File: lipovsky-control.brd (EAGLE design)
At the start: 59 x 32 mm, 31 parts, among them J1 M04-929P, J2 M04-929P, J3 M04-929P, J4 M04-929P, U1 ATTINYX4A8MU, U10 CCR20MA_45V, U2 MIC2288YD5, U3 MIC2288YD5, U7 LTV-816S

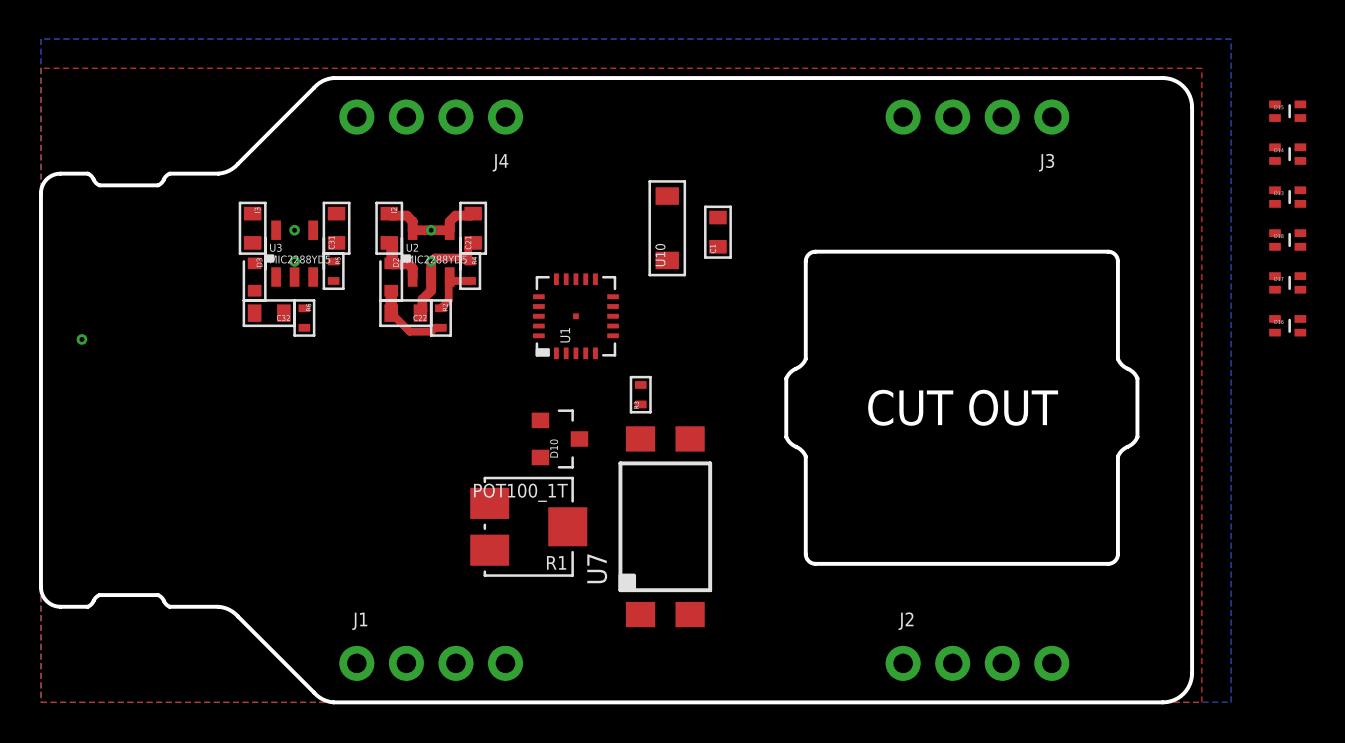
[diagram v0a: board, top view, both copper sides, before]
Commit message: LED matrix
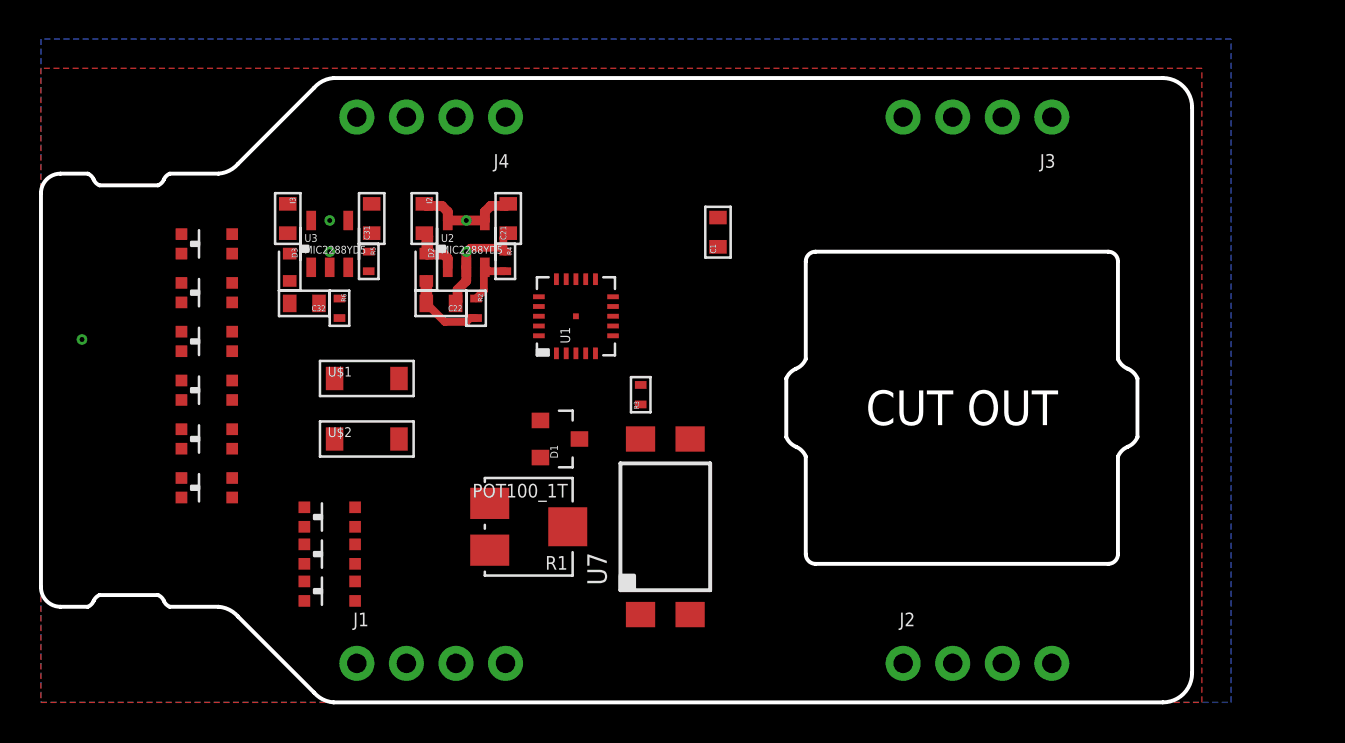
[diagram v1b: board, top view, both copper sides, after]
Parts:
- removed D13, D14, D15, D16, D17, D18: LED_DUALGO, dubec:0603+DUAL
- removed U10: CCR20MA_45V, dubec:SOD-123
- added D101, D102, D103, D104, D105, D106, D4, D5, D6: LED_DUALRG-2, dubec:1206+DUAL
- added U$1, U$2: CCR10MA, dubec:SOD-123
- moved C21 1.87 mm to (23.9, 24.8)
- moved C22 1.87 mm to (20.5, 20.4)
- moved C32 1.87 mm to (13.5, 20.4)
- moved D2 1.87 mm to (19.8, 22.3)
- moved D3 1.87 mm to (12.8, 22.3)
- moved I3 1.87 mm to (12.7, 24.8)
- moved R2 1.87 mm to (22.3, 20.2)
- moved R4 1.87 mm to (23.8, 22.6)
- moved R5 1.87 mm to (16.8, 22.6)
- moved R6 1.87 mm to (15.3, 20.2)
- moved U2 1.87 mm to (21.8, 23.5)
- moved U3 1.87 mm to (14.8, 23.5)
- moved C31 1.87 mm to (16.9, 24.8)
- moved I2 1.87 mm to (19.6, 24.8)
- renumbered D10 to D1
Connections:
- removed net C1: U10.A
- removed net N$12: D16.C1
- removed net N$13: D17.C1
- removed net N$16: D18.C1
- removed net N$2: U10.C
- new net D2: D104.A2, D104.C1, D105.A2, D105.C1, D106.A2, D106.C1
- new net D3: D4.A2, D4.C1, D5.A2, D5.C1, D6.A2, D6.C1
- new net D4: D101.A1, D101.C2, D104.A1, D104.C2, D4.A1, D4.C2
- new net D5: D102.A1, D102.C2, D105.A1, D105.C2, D5.A1, D5.C2
- new net D6: D103.A1, D103.C2, D106.A1, D106.C2, D6.A1, D6.C2
- net D1: now also D101.A2, D101.C1, D102.A2, D102.C1, D103.A2, D103.C1; no longer D13.A2, D13.C1, D14.A2, D14.C1, D15.A2, D15.C1

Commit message: .
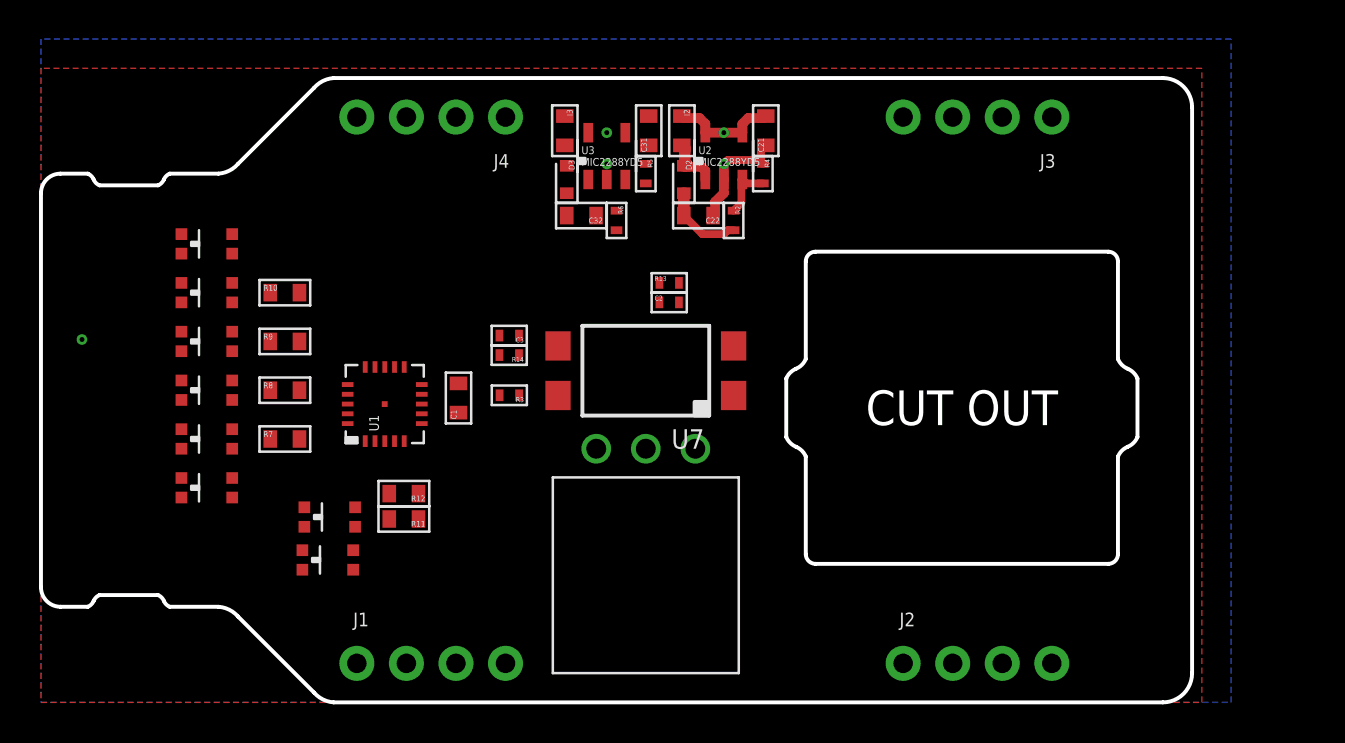
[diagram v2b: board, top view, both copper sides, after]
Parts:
- removed D1: D_ZENER3V, dubec:SOT23-3
- removed D6: LED_DUALRG-2, dubec:1206+DUAL
- removed U$1, U$2: CCR10MA, dubec:SOD-123
- added C2: CAP470N_10V, dubec:0402
- added C3: CAP47N_50V, dubec:0402
- added R10, R11, R12, R7, R8, R9: RES150_10, dubec:0603
- added R13, R14: RES330_16, dubec:0402
- R1: value POT100_1T -> POT5K; device dubec:ST-4EA -> dubec:3296W
- R3: value RES590_16 -> RES330_16
- moved C1 15.8 mm to (21.4, 15.6)
- moved I3 14.9 mm to (26.9, 29.3)
- moved C31 14.9 mm to (31.1, 29.3)
- moved C32 14.9 mm to (27.7, 24.9)
- moved D3 14.9 mm to (26.9, 26.8)
- moved R5 14.9 mm to (31.0, 27.1)
- moved R6 14.9 mm to (29.5, 24.7)
- moved U3 14.9 mm to (29.0, 28.0)
- moved C22 13.9 mm to (33.7, 24.9)
- moved D2 13.9 mm to (33.0, 26.8)
- moved I2 13.9 mm to (32.9, 29.3)
- moved C21 13.9 mm to (37.1, 29.3)
- moved R2 13.9 mm to (35.5, 24.7)
- moved R4 13.9 mm to (37.0, 27.1)
- moved U2 13.9 mm to (35.0, 28.0)
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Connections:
- net N$10 renamed !RESET
- net VCC_REG renamed +8V
- removed net D5: D102.A1, D102.C2, D105.A1, D105.C2, D5.A1, D5.C2
- removed net D6: D103.A1, D103.C2, D106.A1, D106.C2, D6.A1, D6.C2
- removed net N$14: U1.15
- removed net N$15: U1.16
- removed net N$3: U1.5
- removed net SFB: J1.3, U1.4
- removed net VCC: C22.2, D2.C, J4.3, R2.2, R3.2, U1.9
- new net +5V: C1.2, C22.2, D2.C, J4.3, R12.1, R2.2, U1.9, U7.4
- new net D_OVERTEMP: D5.A1, D5.C2, U1.15
- new net D_STATUS: D4.A1, D4.C2, U1.16
- new net FB_ADC: C3.2, R14.1, U1.4
- new net N$2: D4.A2, D4.C1, D5.A2, D5.C1, R11.2, R12.2
- new net S_ADC: C2.1, R13.2, U1.5
- net D1: now also D101.A1, D101.C2, D102.A1, D102.C2, D103.A1, D103.C2, R7.1; no longer D101.A2, D101.C1, D102.A2, D102.C1, D103.A2, D103.C1
- net D2: now also D101.A2, D101.C1, D104.A1, D104.C2, D105.A1, D105.C2, R8.1; no longer D104.A2, D104.C1, D105.A2, D105.C1, D106.A2, D106.C1
- net D3: now also D102.A2, D102.C1, D104.A2, D104.C1, D105.A2, D105.C1, D106.A1, D106.C2, R9.1; no longer D4.A2, D4.C1, D5.A2, D5.C1, D6.A2, D6.C1
- net D4: now also D103.A2, D103.C1, D106.A2, D106.C1, R10.1; no longer D101.A1, D101.C2, D104.A1, D104.C2, D4.A1, D4.C2
- net FB: now also R14.2, R3.2; no longer R1.2
- net N$1: now also R1.WIPER; no longer D1.3, U7.4
- net N$5: now also R7.2
- net N$6: now also R8.2
- net N$7: now also R9.2
- net N$8: now also R10.2
- net S+: now also R13.1
- net S-: now also C1.1, C2.2, C3.1, R1.CW, R11.1; no longer D1.1, R1.3
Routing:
- net VCC: track 4.18 -> 0.00 mm
- net +5V: track 0.00 -> 4.18 mm
